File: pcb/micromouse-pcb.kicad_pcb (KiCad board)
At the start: 2 copper layers, 140 x 100 mm, 40 parts, among them J1_MotorEncoder1 Conn_01x06, J2_MotorEncoder1 Conn_01x06, J3 Conn_01x08, J4 Conn_01x08, Q1 BS170, Q2 TEFT4300, Q3 BS170, Q4 TEFT4300, Q5 BS170, Q6 TEFT4300, Q7 BS170, Q8 TEFT4300, SW1 SW_SPDT, U0 Teensy 4.1, U2 L7805

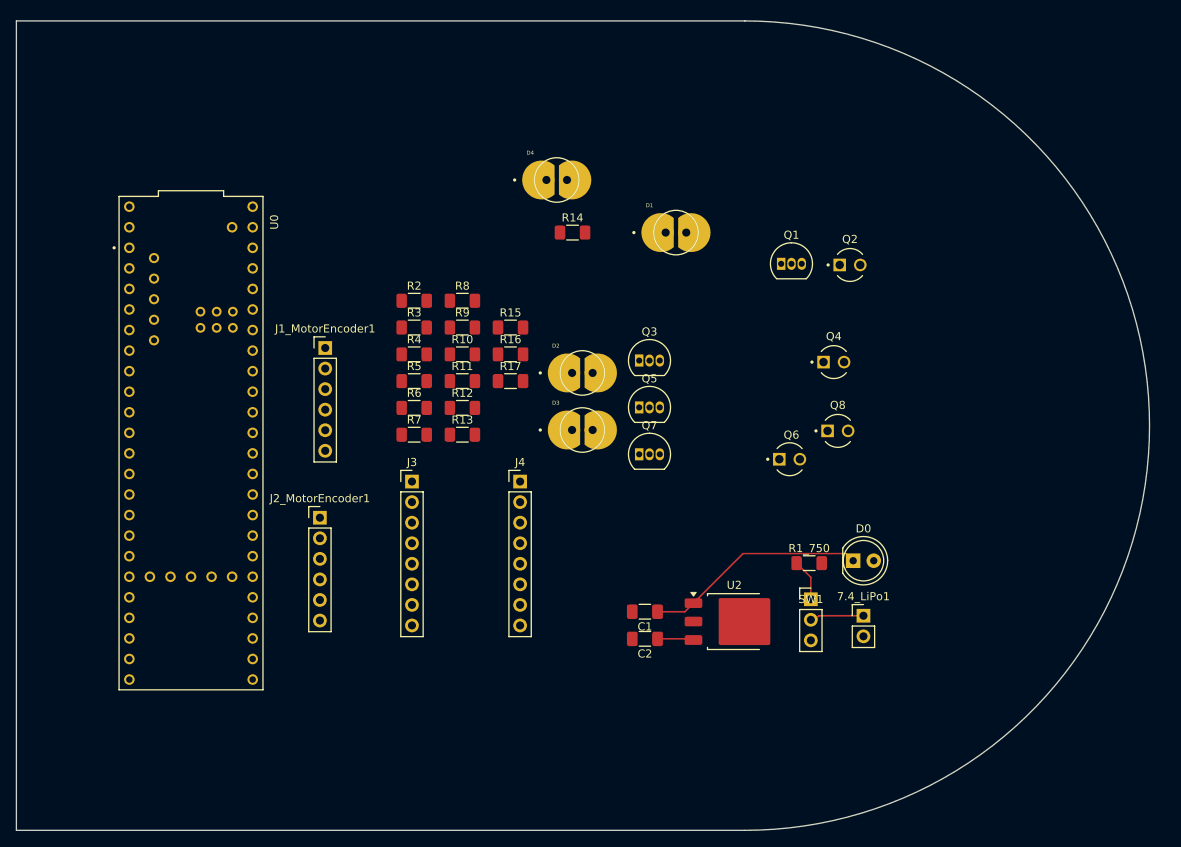
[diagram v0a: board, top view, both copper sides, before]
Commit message: edited pcb
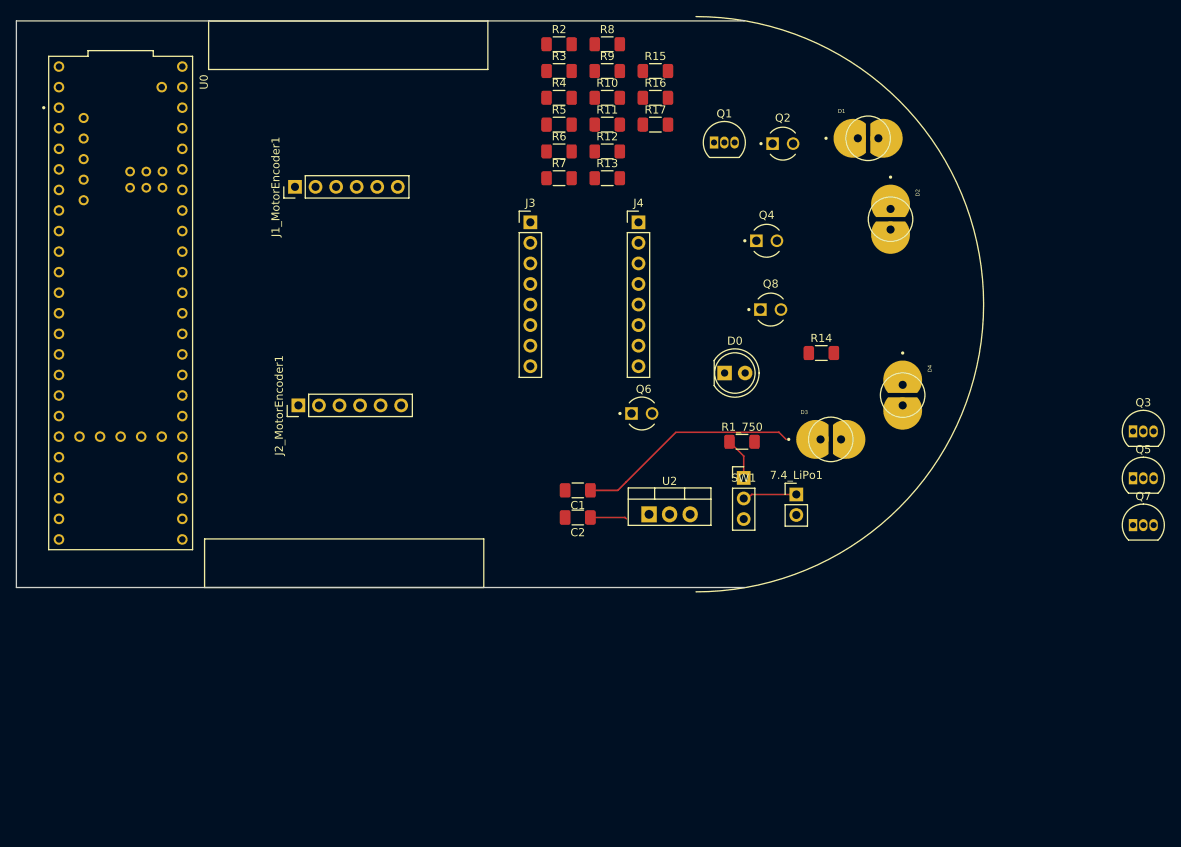
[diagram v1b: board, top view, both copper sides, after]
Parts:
- U2: footprint Package_TO_SOT_SMD:TO-252-3_TabPin2 -> Package_TO_SOT_THT:TO-220-3_Vertical
- moved Q3 61.6 mm to (183.5, 67.7)
- moved Q5 61.6 mm to (183.5, 73.5)
- moved Q7 61.6 mm to (183.5, 79.3)
- moved D4 50.3 mm to (155.0, 63.2), turned to -90 degrees
- moved D2 42.5 mm to (153.5, 41.5), turned to -90 degrees
- moved R11 36.4 mm to (118.5, 29.8)
- moved R15 36.4 mm to (124.5, 23.2)
- moved R17 36.4 mm to (124.5, 29.8)
- moved R8 36.4 mm to (118.5, 19.9)
- moved R9 36.4 mm to (118.5, 23.2)
- moved R10 36.4 mm to (118.5, 26.5)
- moved R12 36.4 mm to (118.5, 33.1)
- moved R13 36.4 mm to (118.5, 36.4)
- moved R16 36.4 mm to (124.5, 26.5)
- moved R2 36.4 mm to (112.5, 19.9)
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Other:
- board size 140 x 100 mm -> 90 x 70 mm
